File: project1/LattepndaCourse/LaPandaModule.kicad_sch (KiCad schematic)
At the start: 10 parts, among them J1 Conn_01x03_Pin

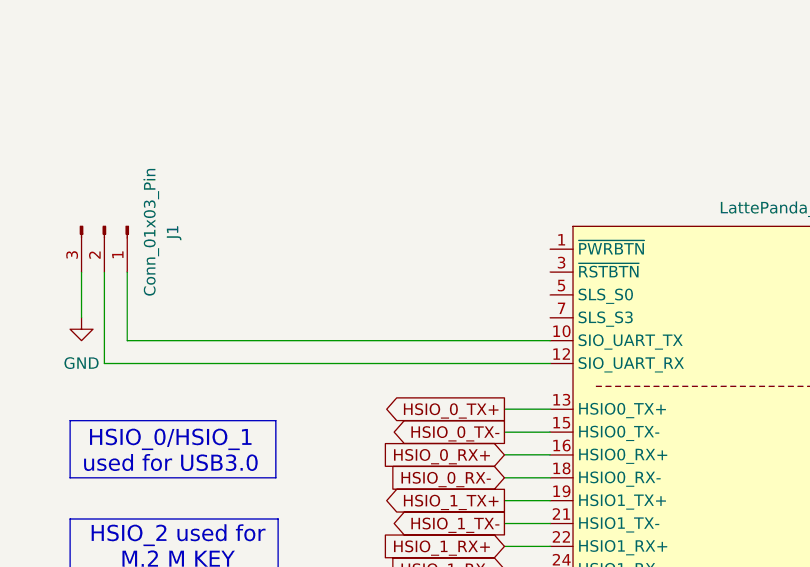
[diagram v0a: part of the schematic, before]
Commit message: power is done
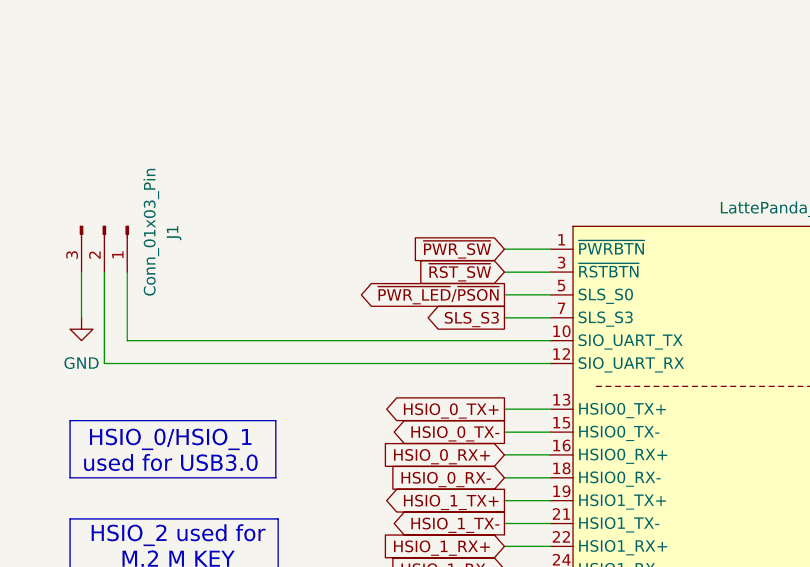
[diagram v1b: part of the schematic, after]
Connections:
- net ~{PWR_SW}: now reaches A1.1 (~{PWRBTN})
- net ~{RST_SW}: now reaches A1.3 (~{RSTBTN})
- net ~{PWR_LED}/~{PSON}: now reaches A1.5 (SLS_S0)
- net SLS_S3: now reaches A1.7 (SLS_S3)
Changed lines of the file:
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@@
 	(wire
 		(pts
+			(xy 250.19 71.12) (xy 255.27 71.12)
+		)
+		(stroke
+			(width 0)
+			(type default)
+		)
+	)
+	(wire
+		(pts
 			(xy 336.55 177.8) (xy 340.36 177.8)
 		)
@@
 	(wire
 		(pts
+			(xy 250.19 68.58) (xy 255.27 68.58)
+		)
+		(stroke
+			(width 0)
+			(type default)
+		)
+	)
+	(wire
+		(pts
 			(xy 250.19 241.3) (xy 255.27 241.3)
 		)
@@
 	(wire
 		(pts
+			(xy 250.19 66.04) (xy 255.27 66.04)
+		)
+		(stroke
+			(width 0)
+			(type default)
+		)
+	)
+	(wire
+		(pts
 			(xy 205.74 78.74) (xy 255.27 78.74)
 		)
@@
 	(wire
 		(pts
+			(xy 250.19 73.66) (xy 255.27 73.66)
+		)
+		(stroke
+			(width 0)
+			(type default)
+		)
+	)
+	(wire
+		(pts
 			(xy 336.55 105.41) (xy 340.36 105.41)
 		)
@@
 		)
 	)
+	(global_label "~{PWR_LED}{slash}~{PSON}"
+		(shape output)
+		(at 250.19 71.12 180)
+		(fields_autoplaced yes)
+		(effects
+			(font
+				(size 1.27 1.27)
+			)
+			(justify right)
+		)
+		(property "Intersheetrefs" "${INTERSHEET_REFS}"
+			(at 232.3277 71.12 0)
+			(hide yes)
+			(show_name no)
+			(do_not_autoplace no)
+			(effects
+				(font
+					(size 1.27 1.27)
+				)
+				(justify right)
+			)
+		)
+	)
 	(global_label "REFCLK4-"
 		(shape output)
@@
 		)
 	)
+	(global_label "~{PWR_SW}"
+		(shape input)
+		(at 250.19 66.04 180)
+		(fields_autoplaced yes)
+		(effects
+			(font
+				(size 1.27 1.27)
+			)
+			(justify right)
+		)
+		(property "Intersheetrefs" "${INTERSHEET_REFS}"
+			(at 239.5849 66.04 0)
+			(hide yes)
+			(show_name no)
+			(do_not_autoplace no)
+			(effects
+				(font
+					(size 1.27 1.27)
+				)
+				(justify right)
+			)
+		)
+	)
 	(global_label "HSIO_1_TX-"
 		(shape output)
@@
 		)
 	)
+	(global_label "~{RST_SW}"
+		(shape input)
+		(at 250.19 68.58 180)
+		(fields_autoplaced yes)
+		(effects
+			(font
+				(size 1.27 1.27)
+			)
+			(justify right)
+		)
+		(property "Intersheetrefs" "${INTERSHEET_REFS}"
+			(at 240.1292 68.58 0)
+			(hide yes)
+			(show_name no)
+			(do_not_autoplace no)
+			(effects
+				(font
+					(size 1.27 1.27)
+				)
+				(justify right)
+			)
+		)
+	)
 	(global_label "UART1_RXD"
 		(shape input)
@@
 			)
 		)
+	)
+	(global_label "SLS_S3"
+		(shape output)
+		(at 250.19 73.66 180)
+		(fields_autoplaced yes)
+		(effects
+			(font
+				(size 1.27 1.27)
+			)
+			(justify right)
+		)
+		(property "Intersheetrefs" "${INTERSHEET_REFS}"
+			(at 240.3711 73.66 0)
+			(hide yes)
+			(show_name no)
+			(do_not_autoplace no)
+			(effects
+				(font
+					(size 1.27 1.27)
+				)
+				(justify right)
+			)
+		)

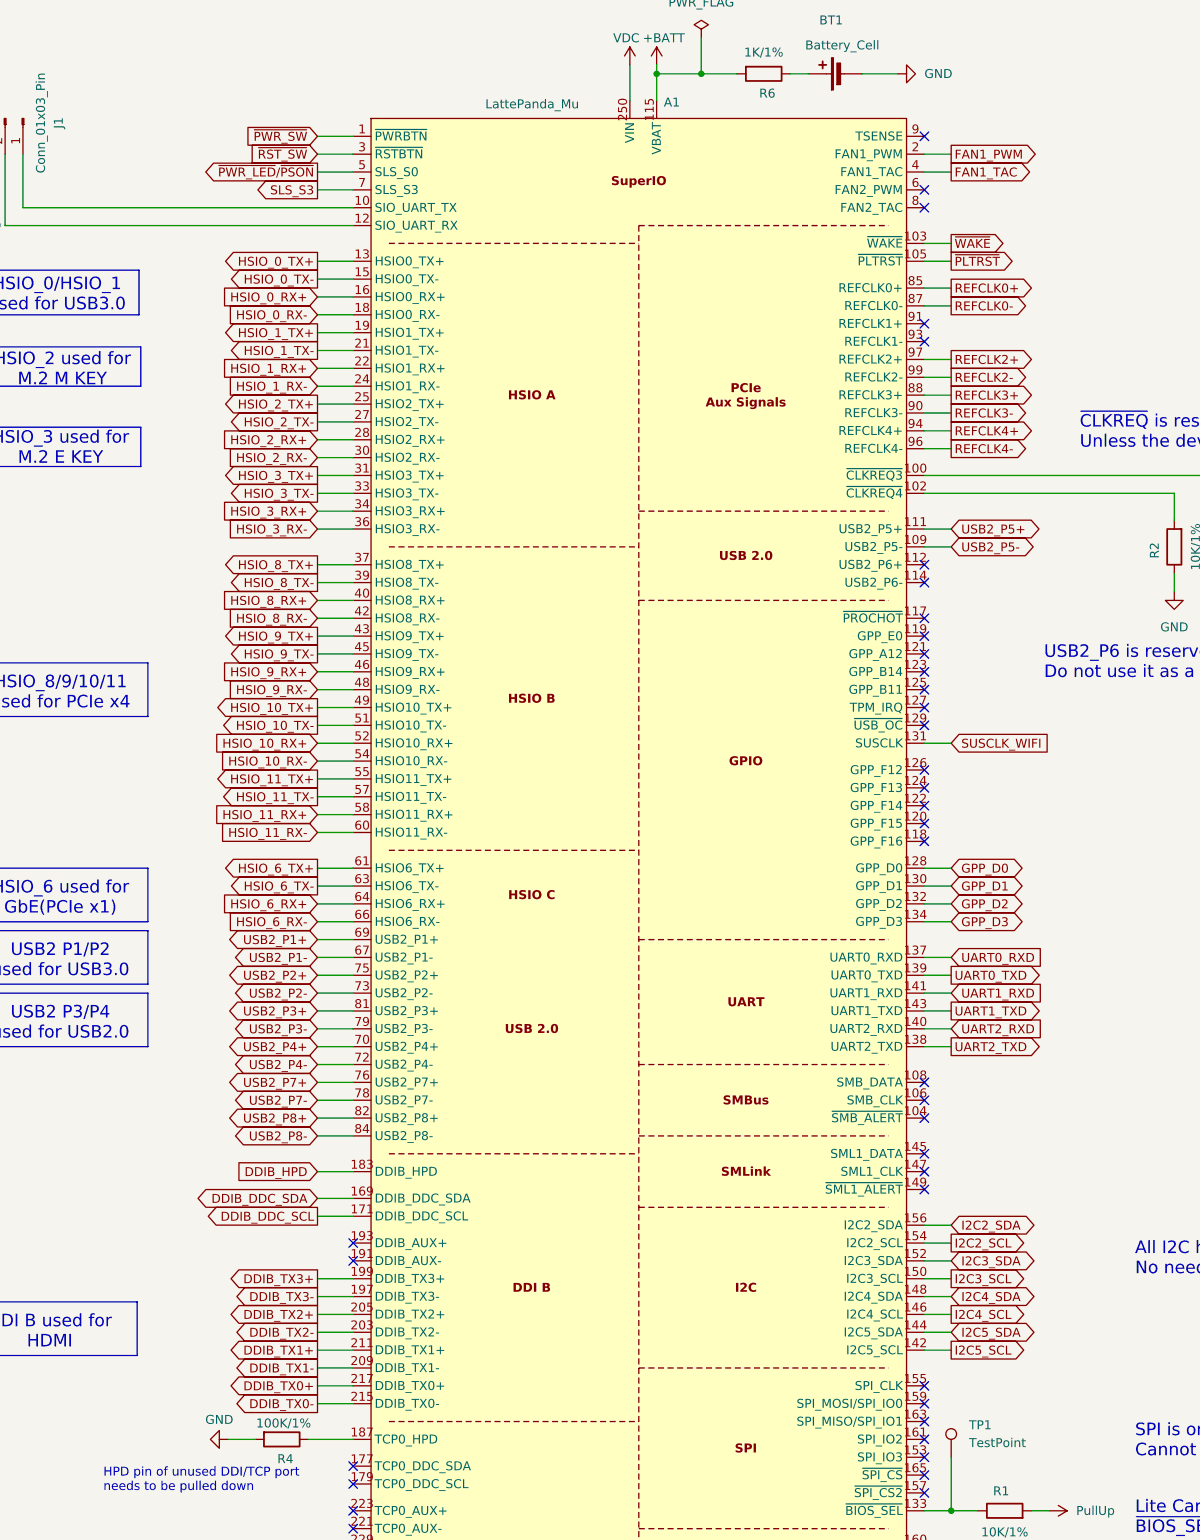
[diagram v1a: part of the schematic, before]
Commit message: Hierachi needs some work
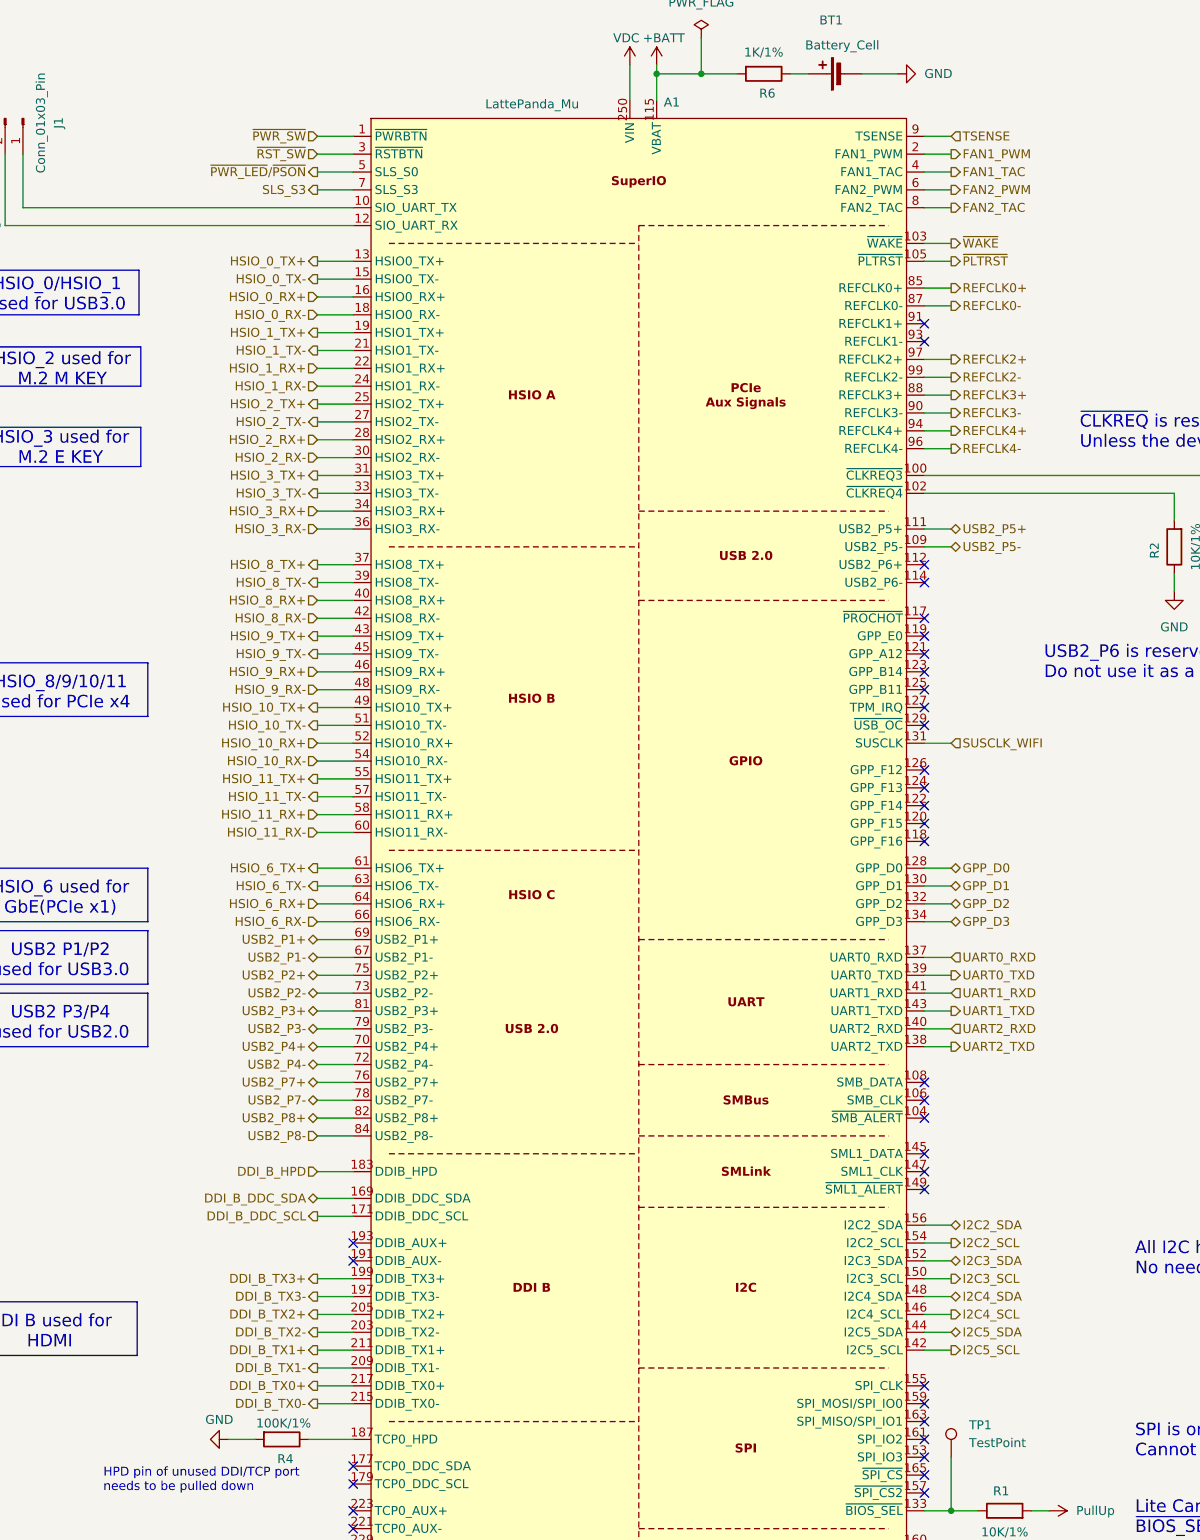
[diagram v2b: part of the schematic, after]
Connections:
- net FAN2_PWM: now reaches A1.6 (FAN2_PWM)
- net FAN2_TAC: now reaches A1.8 (FAN2_TAC)
- net TSENSE: now reaches A1.9 (TSENSE)
- net DDIB_DDC_SCL renamed DDI_B_DDC_SCL
- net DDIB_DDC_SDA renamed DDI_B_DDC_SDA
- net DDIB_HPD renamed DDI_B_HPD
- net DDIB_TX0+ renamed DDI_B_TX0+
- net DDIB_TX0- renamed DDI_B_TX0-
- net DDIB_TX1+ renamed DDI_B_TX1+
- net DDIB_TX1- renamed DDI_B_TX1-
- net DDIB_TX2+ renamed DDI_B_TX2+
- net DDIB_TX2- renamed DDI_B_TX2-
- net DDIB_TX3+ renamed DDI_B_TX3+
- net DDIB_TX3- renamed DDI_B_TX3-
- no-connect marks 80 -> 77
